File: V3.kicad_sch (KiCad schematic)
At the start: 99 parts, among them IC1 TPS62840DLCR","TPS62840DLCR, J1 Conn_01x04, J2 Conn_01x04, J3 FFC2B28-24-G, J4 Conn_01x04, J6 Conn_01x02, J7 Conn_01x02, Q3 FDN304P","FDN304P, Q4 FDN304P","FDN304P, Q6 FDN304P","FDN304P, Q8 SI1308EDL","SI1308EDL, U10 92, U11 BC660KGLAA-I03-SNASA","BC660K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, U12 1042240820","1042240820, U13 92, U14 92, U15 92, U16 92, U17 92, U2 XIAO","102010448, U4 92, U5 92, U6 92, U7 92, U8 92, U9 92

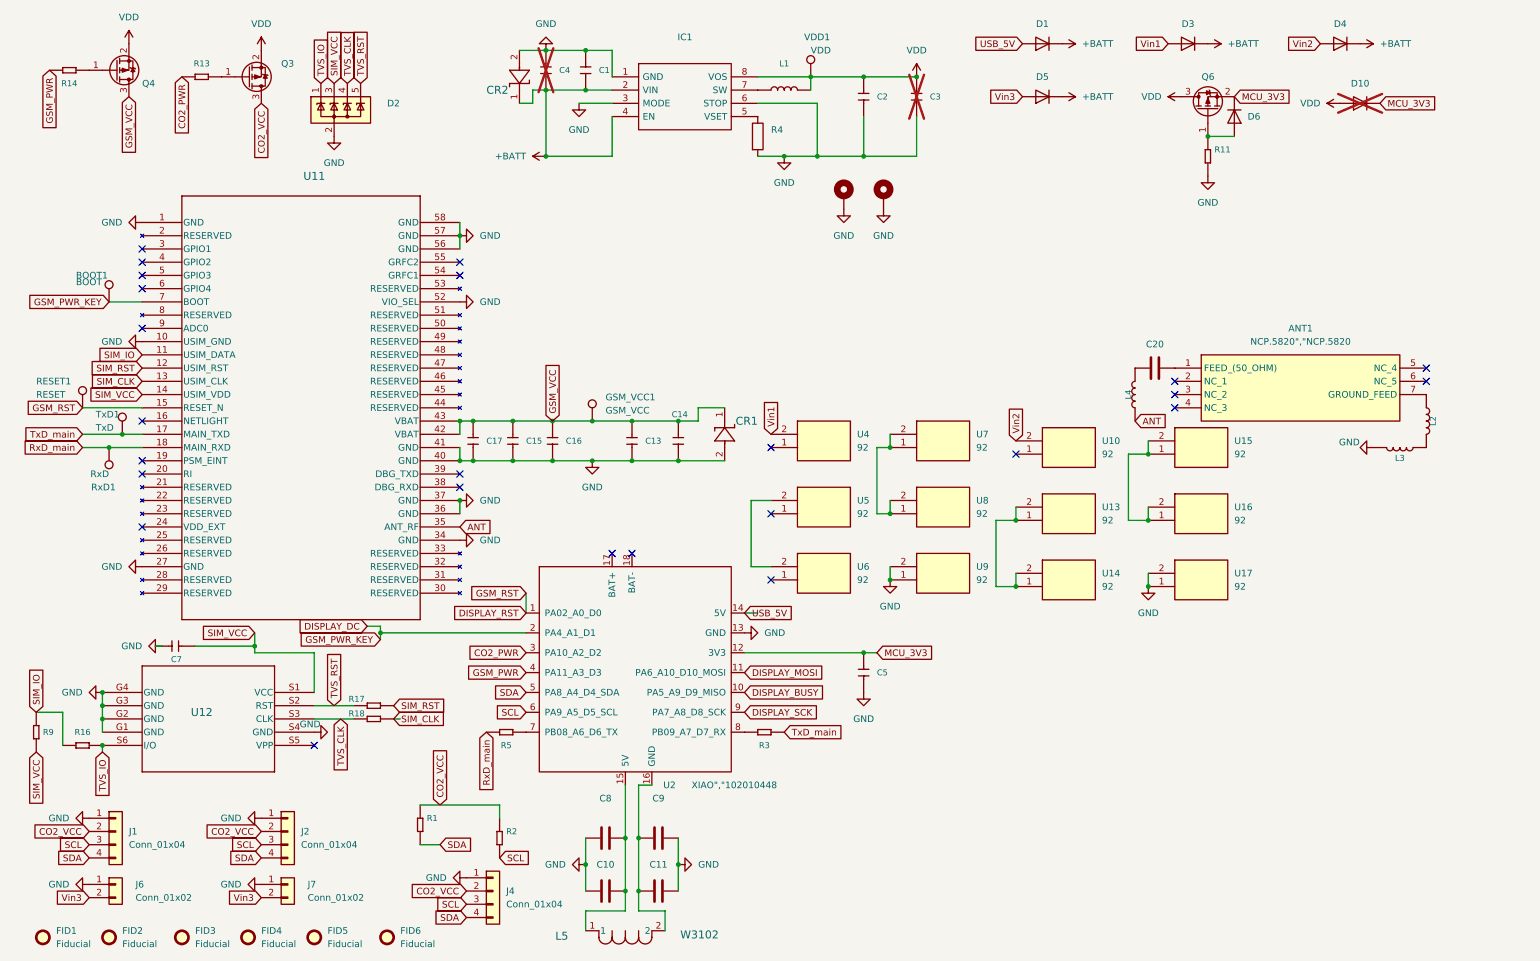
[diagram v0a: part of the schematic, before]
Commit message: revision to review with ideal diode oring
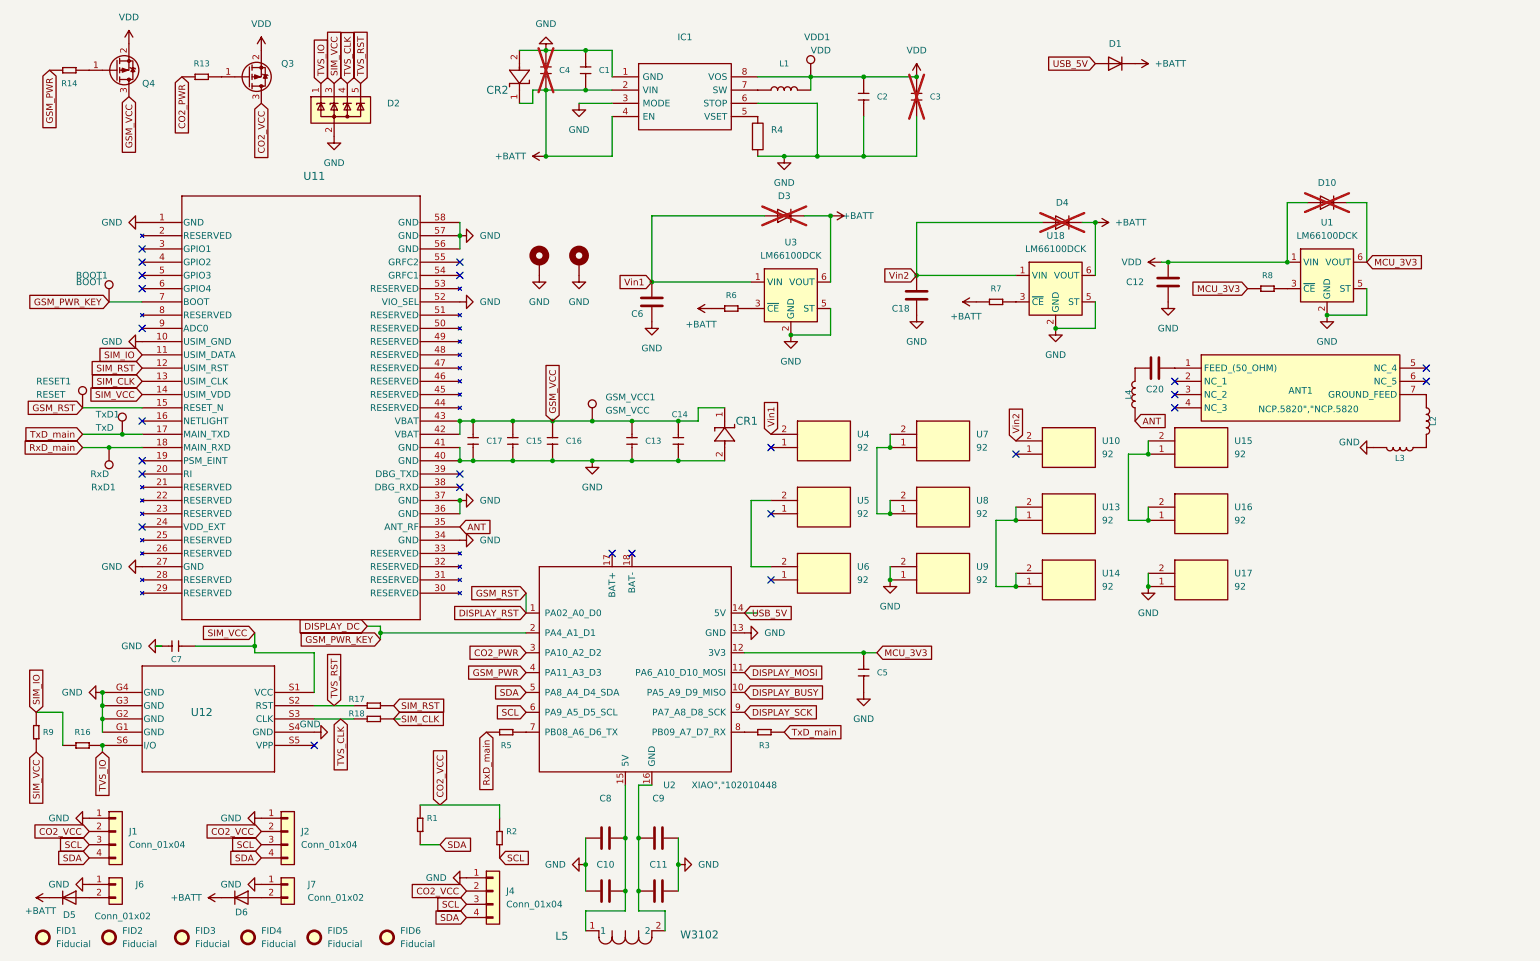
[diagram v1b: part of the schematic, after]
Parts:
- removed Q6: FDN304P","FDN304P, Package_TO_SOT_SMD:SOT-23, symbol Transistor_FET:FDN340P
- removed R11: 100K","RC0603JR-07100KL, kicad_mod:R0603, symbol OPL_Resistor:SMD-RES-10K-5%-1_10W_0603_
- added C12, C18, C6: 1uF",CC0603KRX5R7BB105, kicad_mod:C0603, symbol Device:C
- added R6, R7, R8: 10K","RC0603JR-0710KL, kicad_mod:R0603, symbol OPL_Resistor:SMD-RES-10K-5%-1_10W_0603_
- added U1, U18, U3: LM66100DCK, Package_TO_SOT_SMD:SOT-363_SC-70-6, symbol Power_Management:LM66100DCK
- D3, D4: now not fitted; now left out of the parts list
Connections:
- net +BATT: now also D6.1 (K), R6.1, R7.1, U18.6 (VOUT), U3.6 (VOUT)
- net GND: now also C12.2, C18.1, C6.1, U1.2 (GND), U1.5 (ST), U18.2 (GND), U18.5 (ST), U3.2 (GND), U3.5 (ST)
- net MCU_3V3: now also R8.1, U1.6 (VOUT); no longer D6.1 (K)
- net VDD: now also C12.1, U1.1 (VIN)
- net Vin1: now also C6.2, U3.1 (VIN)
- net Vin2: now also C18.2, U18.1 (VIN)
- net at D6.2 (A): now also J7.2 (Pin_2)
- net Vin3: no longer names the net of D5.2 (A), J6.2 (Pin_2)
- net Vin3: no longer J7.2 (Pin_2)
- new net: R6.2, U3.3 (~{CE})
- new net: R8.2, U1.3 (~{CE})
- new net: R7.2, U18.3 (~{CE})
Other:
- moved on the sheet: D1, D10, D5
